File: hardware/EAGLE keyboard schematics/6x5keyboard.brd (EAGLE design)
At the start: 117.8 x 116.8 mm, 70 parts

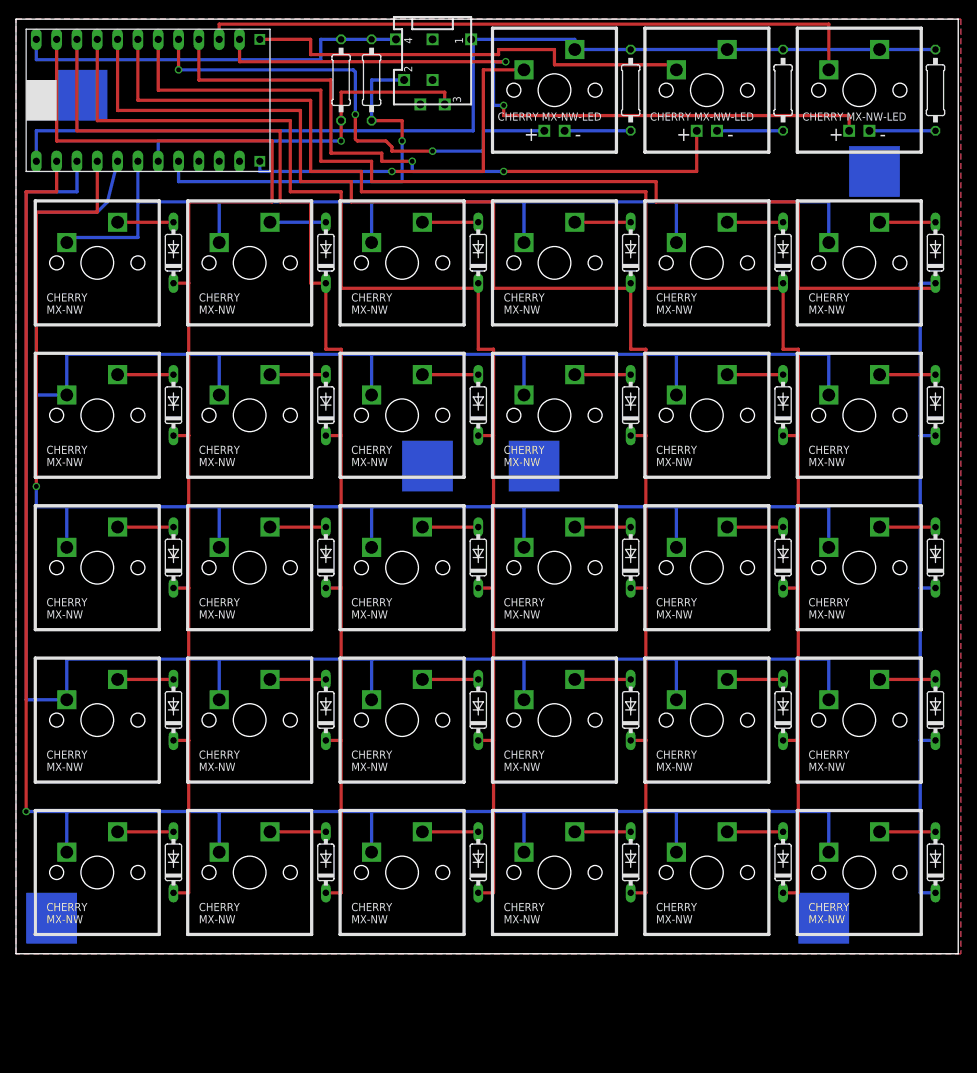
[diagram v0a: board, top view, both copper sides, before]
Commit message: work
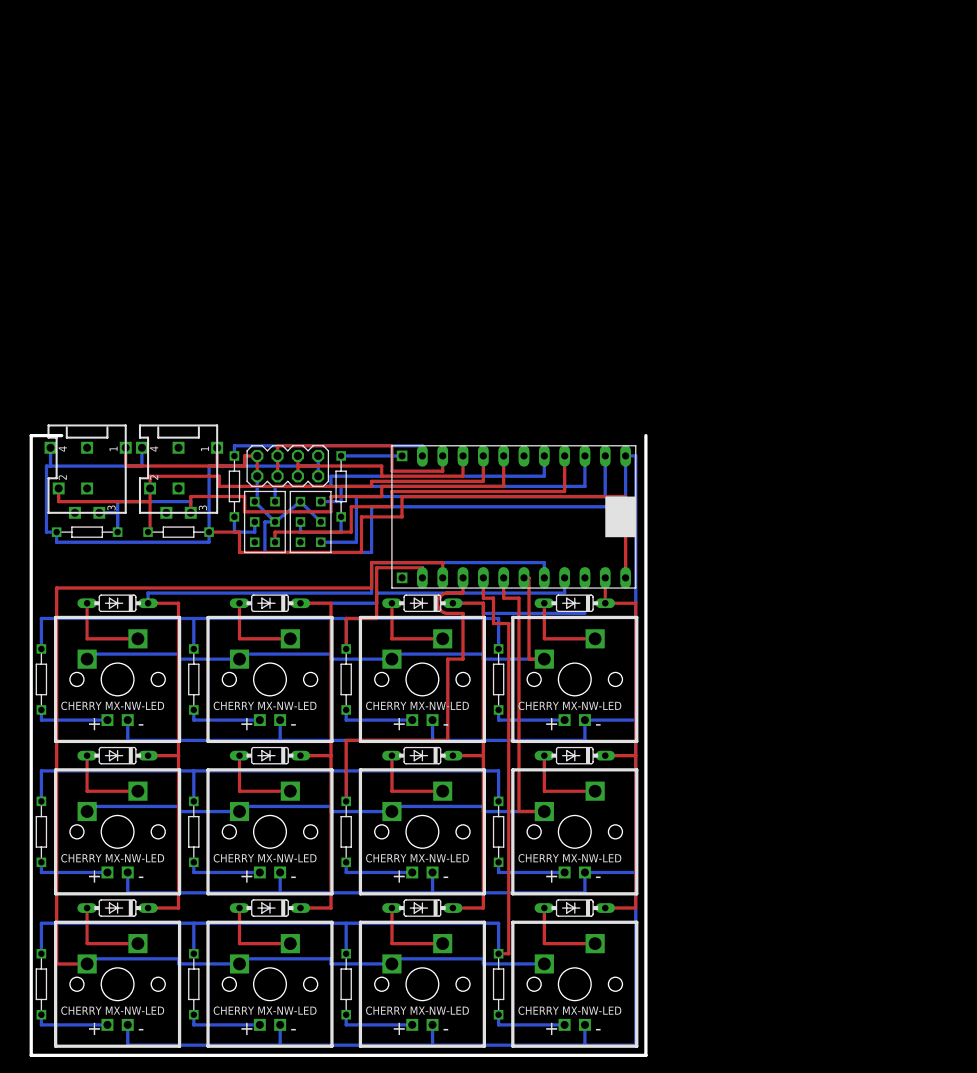
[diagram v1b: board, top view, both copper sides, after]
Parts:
- removed D11, D12, D13, D14, D15, D16, D17, D18, D19, D20, D21, D22, D23, D24, D29, D30, D5, D6: (no value), diode:DO35-7
- removed R1, R2, R3: (no value), rcl:0207/10
- removed R4, R5: 3.3K, resistor:0207/10
- removed U$32, U$33, U$34: CHERRY-MX1A-E1NW-LED, my_parts:CHERRYMX-NN-LED
- added COMM1: SJ-43514_HEADPHONES_3.5MM_X4, my_parts:SJ-43514_HEADPHONES-3.5MM_X4
- added SV1: (no value), con-lstb:MA04-2
- U$1, U$10, U$2, U$25, U$26, U$27, U$28, U$3, U$4, U$7, U$8, U$9: value CHERRY-MX1A-E1NW -> CHERRY-MX1A-E1NW-LED; device my_parts:CHERRYMX-NN -> my_parts:CHERRYMX-NN-LED
- U$11, U$12, U$13, U$14, U$15, U$16, U$17, U$18, U$19, U$20, U$21, U$22, U$29, U$30, U$5, U$6: value CHERRY-MX1A-E1NW -> RESISTORBIGPAD; device my_parts:CHERRYMX-NN -> my_parts:RESISTORBIGPAD
- U$23, U$24: value CHERRY-MX1A-E1NW -> NKK_GW_SERIES; device my_parts:CHERRYMX-NN -> my_parts:NKK_GW_SERIES
- moved U$5 98.1 mm to (4.45, 10.2), turned to 90 degrees
- moved U$6 98.1 mm to (23.5, 10.2), turned to 90 degrees
- moved U$11 84.2 mm to (42.5, 10.2), turned to 90 degrees
- moved U$12 84.2 mm to (61.6, 10.2), turned to 90 degrees
- moved U$24 72.9 mm to (38.1, 67.9), turned to 180 degrees
- moved U$30 70.5 mm to (41.9, 72.4), turned to 90 degrees
- moved U$18 68.5 mm to (42.5, 48.3), turned to 90 degrees
- moved U$31 66.1 mm to (61.0, 68.6), turned to 270 degrees
- moved U$29 65.3 mm to (28.6, 72.4), turned to 90 degrees
- moved U$16 64.3 mm to (4.45, 29.2), turned to 90 degrees
- moved U$22 63.0 mm to (10.2, 66.7), turned to 180 degrees
- moved U$23 60.5 mm to (32.4, 67.9), turned to 180 degrees
- moved COMM 60.1 mm to (21.6, 77.2)
- moved U$10 52.1 mm to (71.1, 29.2)
- moved U$25 52.1 mm to (14.0, 48.3)
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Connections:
- removed net N$43: R2.2, U$33.LED-
- removed net N$44: R3.2, U$34.LED-
- removed net N$46: U$31.PB5, U$33.LED+
- removed net N$47: U$31.PB6, U$34.LED+
- removed net N$48: U$31.PB4, U$32.SIDE
- removed net N$53: COMM.2, R4.1, U$31.PD1
- removed net N$54: U$31.PD7, U$32.LED+
- new net VCC: COMM.4, COMM1.4, SV1.7, SV1.8, U$21.P$1, U$22.P$2, U$31.VCC
- net GND: now also COMM1.1, SV1.1, SV1.2, U$1.LED-, U$10.LED-, U$2.LED-, U$23.P$2, U$23.P$6, U$24.P$2, U$24.P$6, U$25.LED-, U$26.LED-, U$27.LED-, U$28.LED-, U$3.LED-, U$4.LED-, U$7.LED-, U$8.LED-, U$9.LED-; no longer R1.1, R2.1, R3.1, U$32.UP, U$33.UP, U$34.UP
- net N$11: now also U$11.P$1, U$3.LED+; no longer D11.A, U$11.UP
- net N$12: now also U$1.LED+, U$6.P$1; no longer D12.A, U$12.UP
- net N$13: now also U$2.LED+, U$5.P$1; no longer D13.A, U$13.UP
- net N$14: now also U$30.P$2, U$31.PC7; no longer D14.A, U$14.UP
- net N$15: now also U$24.P$5, U$30.P$1; no longer D15.A, U$15.UP
- net N$16: now also COMM.2, COMM1.2, U$21.P$2, U$31.PD1; no longer D16.A, U$16.UP
- net N$17: now also U$29.P$2, U$31.PC6; no longer D17.A, U$17.UP
- net N$18: now also U$10.LED+, U$13.P$1; no longer D18.A, U$18.UP
- net N$19: now also U$14.P$1, U$9.LED+; no longer D19.A, U$19.UP
- net N$20: now also U$15.P$1, U$8.LED+; no longer D20.A, U$20.UP
- net N$21: now also U$16.P$1, U$7.LED+; no longer D21.A, U$21.UP
- net N$22: now also U$24.P$1, U$31.PB0; no longer D22.A, U$22.UP
- net N$23: now also U$17.P$1, U$28.LED+; no longer D23.A, U$23.UP
- net N$24: now also U$18.P$1, U$27.LED+; no longer D24.A, U$24.UP
- net N$29: now also U$19.P$1, U$26.LED+; no longer D29.A, U$29.UP
- net N$30: now also U$20.P$1, U$25.LED+; no longer D30.A, U$30.UP
- net N$31: now also U$31.PF5; no longer D13.C, D19.C, U$31.PF0
- net N$32: now also U$31.PF4; no longer D14.C, D20.C, U$31.PF1
- net N$33: now also U$31.PF1; no longer D15.C, D21.C, U$31.PF4
- net N$34: now also U$31.PF0; no longer D16.C, D22.C, U$31.PF5
- net N$35: now also U$24.P$3, U$31.PB1; no longer D11.C, D17.C, D23.C, D29.C, D5.C, U$31.PF6
- net N$36: now also U$23.P$1, U$31.PB2; no longer D12.C, D18.C, D24.C, D30.C, D6.C, U$31.PF7
- net N$37: now also SV1.3, SV1.4, U$31.PD3; no longer U$19.SIDE, U$20.SIDE, U$21.SIDE, U$22.SIDE, U$23.SIDE, U$24.SIDE, U$31.PB1
- net N$38: now also U$31.PB4; no longer U$31.PB2, U$5.SIDE, U$6.SIDE
- net N$39: now also U$31.PF7; no longer U$11.SIDE, U$12.SIDE, U$31.PB3
- net N$40: now also U$31.PF6; no longer U$29.SIDE, U$30.SIDE, U$31.PB7
- net N$41: now also SV1.5, SV1.6, U$31.PD2; no longer U$13.SIDE, U$14.SIDE, U$15.SIDE, U$16.SIDE, U$17.SIDE, U$18.SIDE, U$31.PB0
- net N$42: now also U$23.P$3, U$31.PB3; no longer R1.2, U$32.LED-
- net N$49: now also U$11.P$2, U$12.P$2, U$31.PB6, U$5.P$2, U$6.P$2; no longer U$31.PD6, U$33.SIDE
- net N$5: now also U$12.P$1, U$4.LED+; no longer D5.A, U$5.UP
- net N$50: now also U$13.P$2, U$14.P$2, U$15.P$2, U$16.P$2, U$31.PB5; no longer U$31.PC7, U$34.SIDE
- net N$51: now also U$17.P$2, U$18.P$2, U$19.P$2, U$20.P$2, U$31.PD7; no longer COMM.4, R4.2, R5.1, U$31.VCC
- net N$52: now also COMM1.3, U$22.P$1; no longer R5.2
- net N$6: now also U$23.P$5, U$29.P$1; no longer D6.A, U$6.UP
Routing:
- net GND: track 129.2 -> 397.7 mm
- net N$41: track 215.9 -> 27.0 mm, vias 1 -> 0
- net N$37: track 204.5 -> 29.5 mm
- net N$36: track 214.6 -> 47.0 mm
- net N$35: track 198.1 -> 38.7 mm
- net VCC: track 0.00 -> 143.8 mm
- net N$34: track 181.6 -> 52.7 mm
- net N$33: track 165.1 -> 67.3 mm
- net N$54: track 90.7 -> 0.00 mm, vias 2 -> 0
- net N$48: track 83.8 -> 0.00 mm
- net N$46: track 83.8 -> 0.00 mm, vias 2 -> 0
- net N$50: track 47.0 -> 119.8 mm, vias 1 -> 0
- net N$39: track 167.1 -> 95.2 mm
- net N$49: track 57.2 -> 123.8 mm
- net N$32: track 147.3 -> 85.7 mm
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- removed copper zone on layer 1, net GND
- removed copper zone on layer 16, net GND
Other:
- board size 117.8 x 116.8 mm -> 76.8 x 77.5 mm
